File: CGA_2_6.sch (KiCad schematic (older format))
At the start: 11 parts, among them U24 74LS244, U32 74LS166, U33 27C256, U34 74LS273, U35 74LS273, U36 74LS244, U37 74LS374, U39 74LS174, U68 74LS86, U7 74LS166

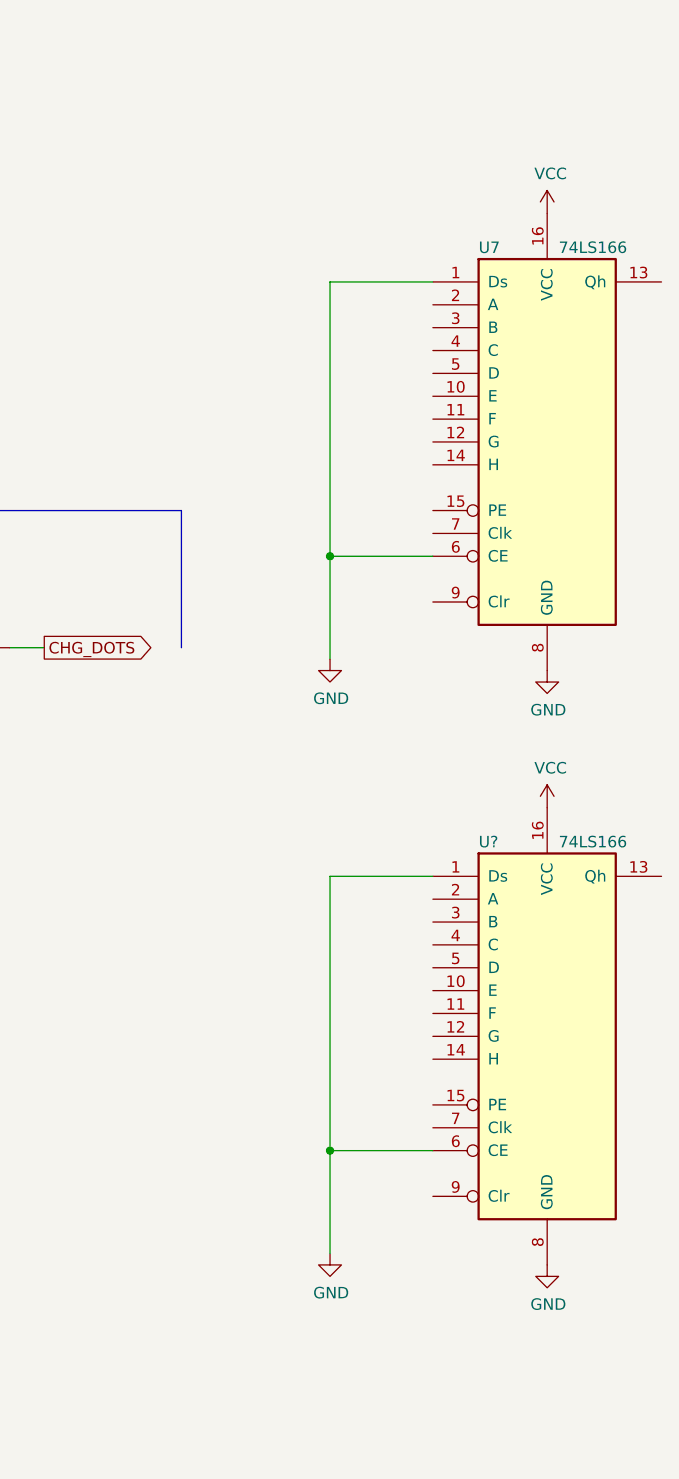
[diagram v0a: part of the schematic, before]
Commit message: More sheet 2
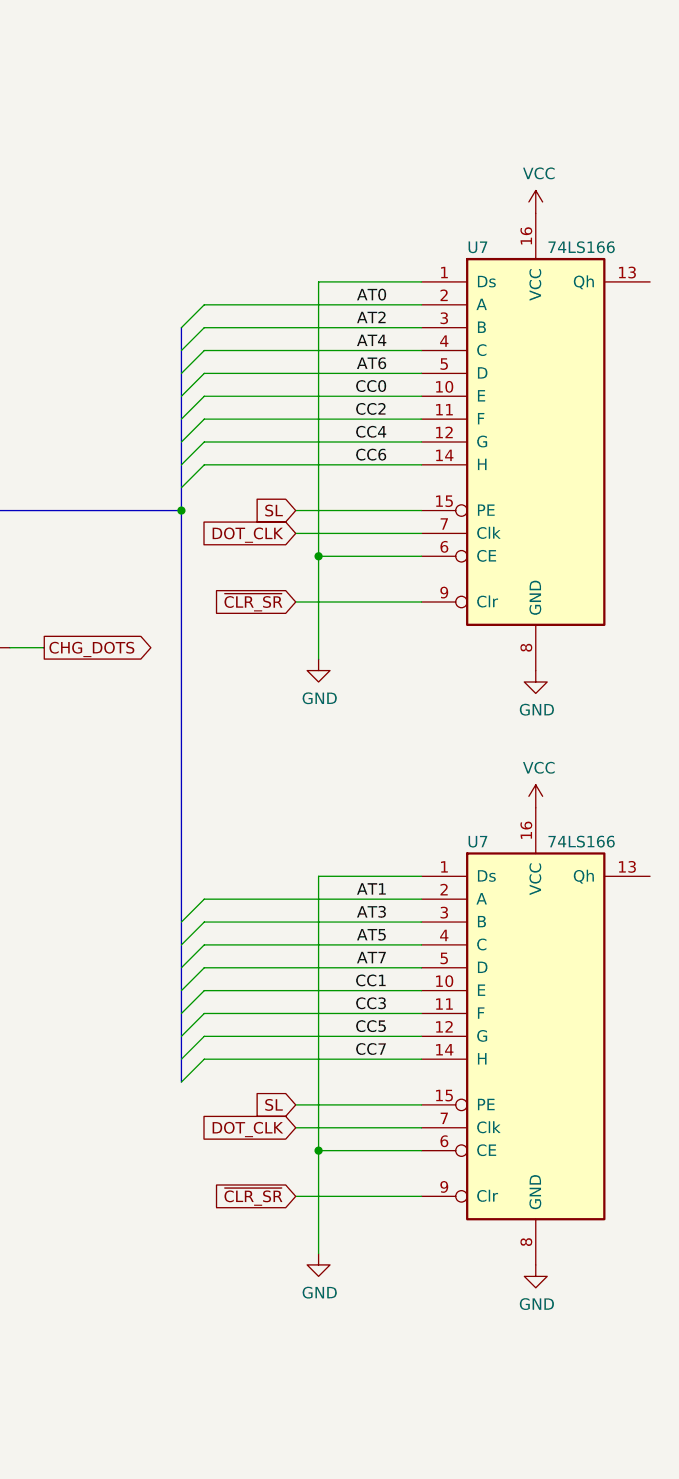
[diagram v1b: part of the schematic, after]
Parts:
- gave numbers to parts that had none: 1
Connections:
- net AT0: now also U7.2 (A)
- net AT1: now also U7.2 (A)
- net AT2: now also U7.3 (B)
- net AT3: now also U7.3 (B)
- net AT4: now also U7.4 (C)
- net AT5: now also U7.4 (C)
- net AT6: now also U7.5 (D)
- net AT7: now also U7.5 (D)
- net CC0: now also U7.10 (E)
- net CC1: now also U7.10 (E)
- net CC2: now also U7.11 (F)
- net CC3: now also U7.11 (F)
- net CC4: now also U7.12 (G)
- net CC5: now also U7.12 (G)
- net CC6: now also U7.14 (H)
- net CC7: now also U7.14 (H)
- net DOT_CLK: now also U7.7 (Clk), U7.7 (Clk)
- net SL: now also U7.15 (PE), U7.15 (PE)
- net ~CLR_SR: now also U7.9 (Clr), U7.9 (Clr)
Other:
- moved on the sheet: U7
